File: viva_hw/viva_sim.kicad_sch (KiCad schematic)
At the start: 18 parts, among them U3 Opamp_Dual, U4 Opamp_Dual

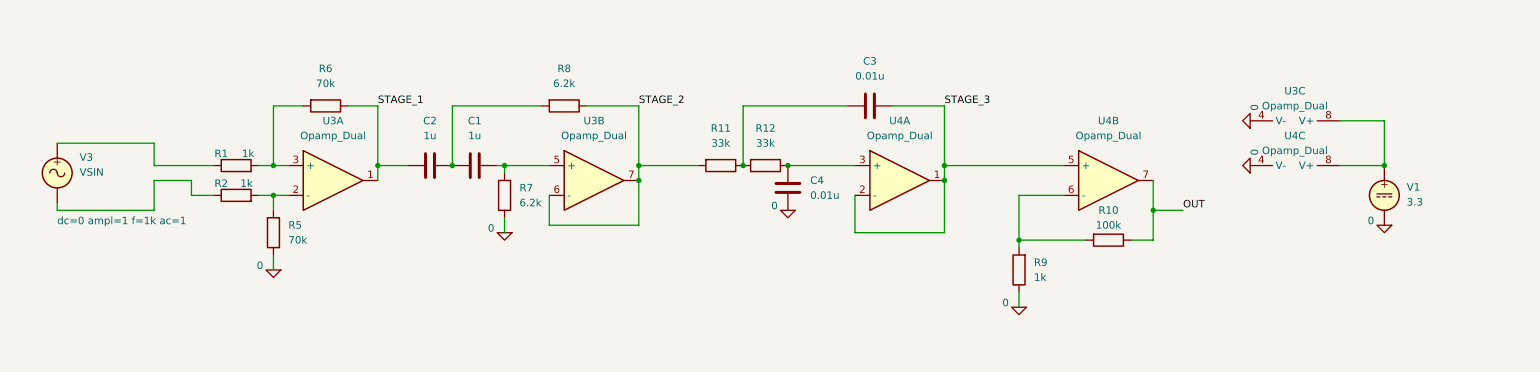
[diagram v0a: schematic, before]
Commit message: feat: emg progress
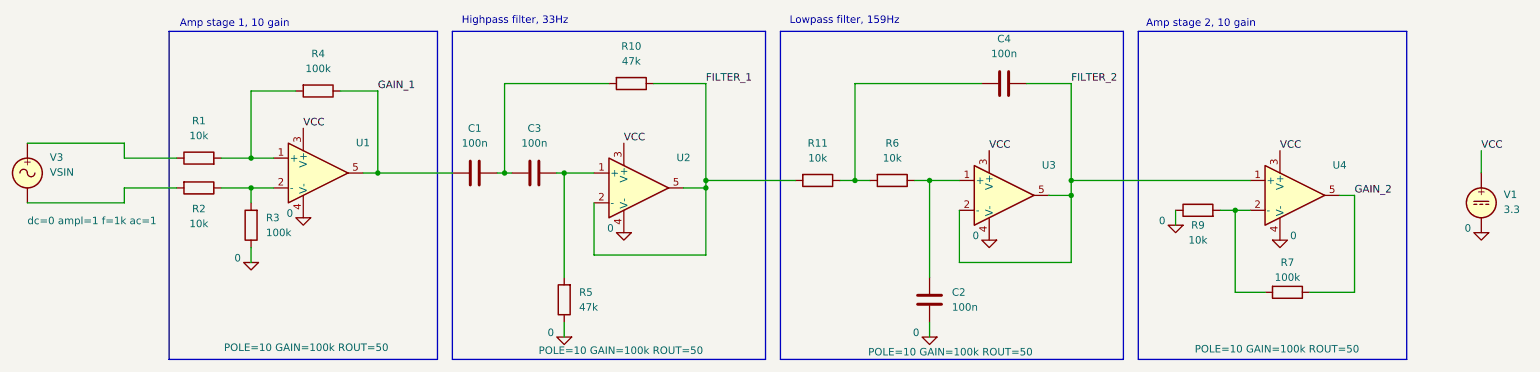
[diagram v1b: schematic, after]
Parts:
- removed R12: 33k, symbol Device:R
- removed R8: 6.2k, symbol Device:R
- removed U3, U4: Opamp_Dual, symbol Device:Opamp_Dual
- added R3, R4: 100k, symbol Device:R
- added U1, U2, U3, U4: ${SIM.PARAMS}, symbol Simulation_SPICE:OPAMP
- C1, C2: value 1u -> 100n
- C3, C4: value 0.01u -> 100n
- R1, R2, R9: value 1k -> 10k
- R10: value 100k -> 47k
- R11: value 33k -> 10k
- R5: value 70k -> 47k
- R6: value 70k -> 10k
- R7: value 6.2k -> 100k
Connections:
- net STAGE_2 is gone; now on net FILTER_1: R11.2
- net STAGE_3 is gone; now on an unnamed net: C3.2
- net 0: now also C2.2, R3.1, U1.4 (V-), U2.4 (V-), U3.4 (V-), U4.4 (V-); no longer C4.1, R7.1
- net FILTER_2: now reaches C4.2
- net FILTER_2: now also U3.2 (-), U3.5, U4.1 (+)
- net at C3.1: now also C1.2, R10.2; no longer R11.1
- net GAIN_1: now reaches C1.1
- net GAIN_1: now also R4.1, U1.5; no longer C2.2
- net at R7.2: now also R9.2, U4.2 (-); no longer C1.2
- net VCC: now reaches V1.1
- net VCC: now also U1.3 (V+), U2.3 (V+), U3.3 (V+), U4.3 (V+)
- net at R1.2: now also R4.2, U1.1 (+); no longer R6.2
- net at R2.1: now also R3.2, U1.2 (-); no longer V3.2
- net at R5.2: now also U2.1 (+); no longer R2.2
- net OUT renamed FILTER_1
- net FILTER_1: now also U2.2 (-), U2.5
- net STAGE_1: no longer names the net of C2.1, R6.1
- net STAGE_1: now also U3.1 (+)
- new net: C4.1, R11.1, R6.2
- new net: R2.2, V3.2
- new net GAIN_2: R7.1, U4.5
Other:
- note added: "Amp stage 1, 10 gain"
- note added: "Amp stage 2, 10 gain"
- note added: "Highpass filter, 33Hz"
- note added: "Lowpass filter, 159Hz"
- moved on the sheet: V1, V3
